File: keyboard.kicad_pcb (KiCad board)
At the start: 2 copper layers, 202.5 x 88.2 mm, 73 parts, among them SW1 SW_SPDT, U1 nice_nano

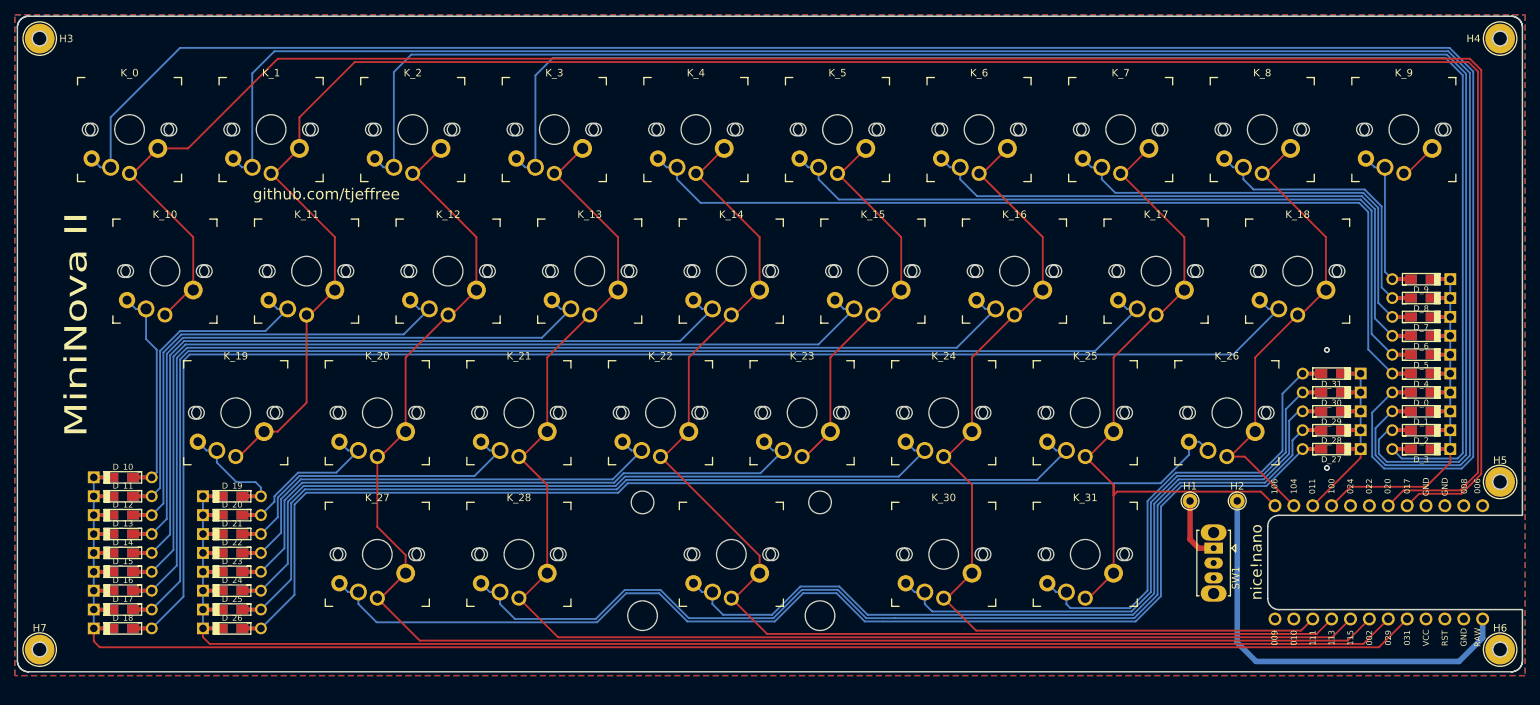
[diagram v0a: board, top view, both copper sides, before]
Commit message: Cut corner version
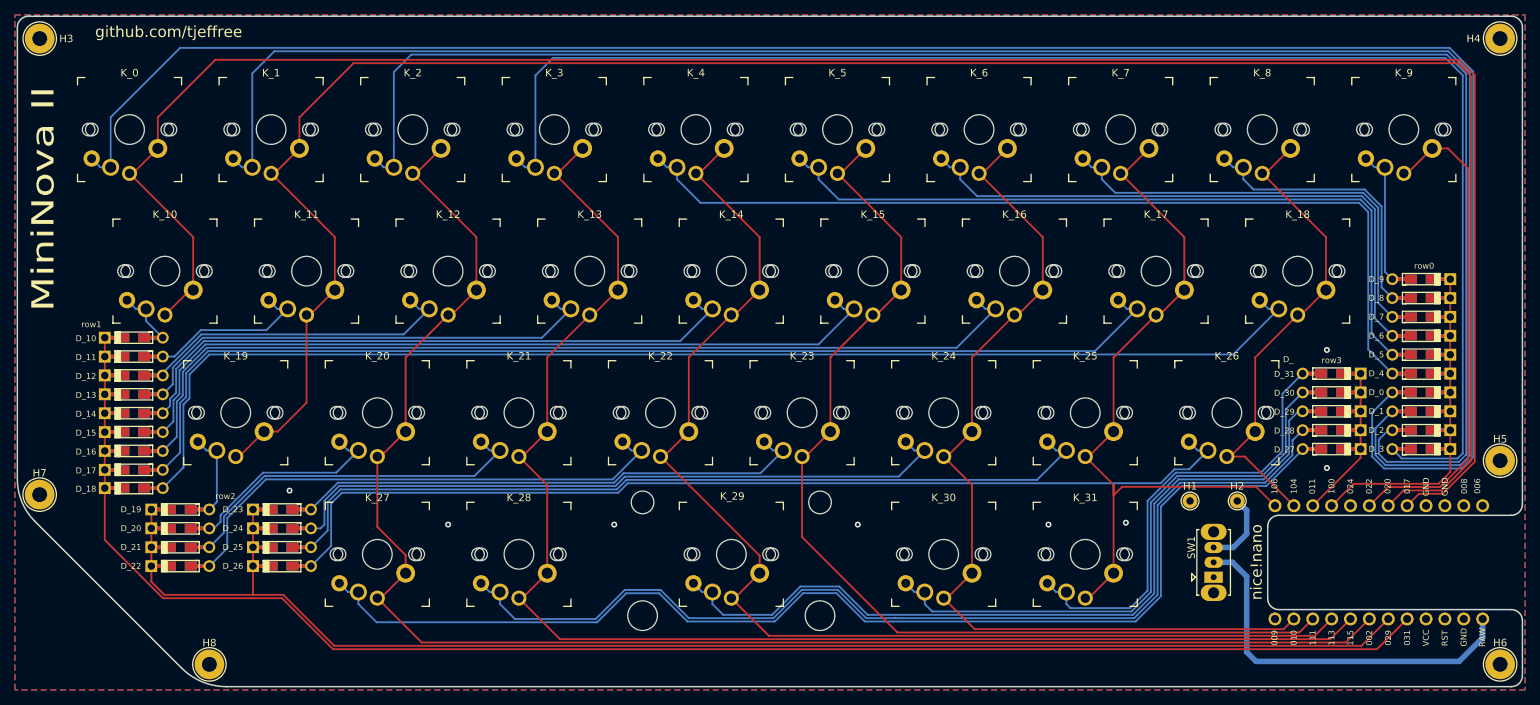
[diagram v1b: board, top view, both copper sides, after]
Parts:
- added H8: Mnt, TestPoint:TestPoint_THTPad_D4.0mm_Drill2.0mm, F.Cu at (54.8, 123.0)
- moved H7 20.8 mm to (31.9, 100.1)
- moved D_18 18.9 mm to (44.6, 99.2)
- moved D_10 18.9 mm to (44.6, 79.0)
- moved D_12 18.9 mm to (44.6, 84.1)
- moved D_14 18.9 mm to (44.6, 89.2)
- moved D_16 18.9 mm to (44.6, 94.2)
- moved D_11 18.9 mm to (44.6, 81.5)
- moved D_13 18.9 mm to (44.6, 86.6)
- moved D_15 18.9 mm to (44.6, 91.7)
- moved D_17 18.9 mm to (44.6, 96.8)
- moved D_24 10.8 mm to (64.5, 104.6)
- moved D_26 10.8 mm to (64.5, 109.7)
- moved D_23 10.8 mm to (64.5, 102.1)
- moved D_25 10.8 mm to (64.5, 107.2)
- moved D_19 7.17 mm to (50.8, 102.1)
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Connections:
- H1 pad 1: Net-(H1-Pad1) -> /GND
- H2 pad 1: Net-(H2-Pad1) -> /BATIN
- SW1 pad 1: Net-(H1-Pad1) -> unconnected-(SW1-Pad1)
- SW1 pad 2: /GND -> /BATIN
- SW1 pad 3: unconnected-(SW1-Pad3) -> /BATIN
- U1 pad 14: unconnected-(U1-Pad14) -> col6
- U1 pad 15: col6 -> col5
- U1 pad 24: Net-(H2-Pad1) -> /BATIN
- U1 pad 7: unconnected-(U1-Pad7) -> col9
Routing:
- net col5: track 52.9 -> 138.5 mm
- net /BATIN: track 0.00 -> 61.7 mm
- net col9: track 5.20 -> 66.1 mm
- net Net-(H2-Pad1): track 57.0 -> 0.00 mm
- net Net-(D_18-Pad2): track 191.1 -> 170.0 mm
- net Net-(D_15-Pad2): track 127.4 -> 106.5 mm
- net Net-(D_16-Pad2): track 148.7 -> 127.7 mm
- net Net-(D_13-Pad2): track 85.0 -> 64.0 mm
- net Net-(D_17-Pad2): track 169.9 -> 148.9 mm
- net Net-(D_14-Pad2): track 106.2 -> 85.2 mm
- net Net-(D_12-Pad2): track 63.8 -> 42.8 mm
- net Net-(D_11-Pad2): track 42.6 -> 22.5 mm
- net Net-(D_10-Pad2): track 26.6 -> 7.85 mm
- net Net-(D_25-Pad2): track 126.3 -> 112.3 mm
- net Net-(D_23-Pad2): track 83.8 -> 69.9 mm
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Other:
- board size 202.5 x 88.2 mm -> 202.5 x 90.2 mm
- board text added: "Bat_GND"
- board text added: "Bat_PWR"
- board text added: "D_"
- board text added: "K_29"
- board text added: "row0"
- board text added: "row1"
- board text added: "row2"
- board text added: "row3"
